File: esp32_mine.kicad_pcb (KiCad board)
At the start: 4 copper layers, 100 x 100 mm, 106 parts, among them J1 USB_C_Receptacle_USB2.0_14P, J3 GPIO, M1 PinHeader_1x02_P2.54mm_Vertic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, M2 PinHeader_1x02_P2.54mm_Vertic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, M3 PinHeader_1x02_P2.54mm_Vertic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, M4 PinHeader_1x02_P2.54mm_Vertic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, Q1 AO3401A, Q2 Q_NMOS_GSD, Q3 Q_NMOS_GSD, Q4 Q_NMOS_GSD, Q5 Q_NMOS_GSD, U1 ESP32-S3, U2 W25Q128JVS, U3 MCP73831-2-OT, U4 BNO055, U5 BMP280, U6 NUP2202, U7 RT9701, Y1 32.768 kHz, Y2 40MHz(10ppm), Y3 32.768 kHz

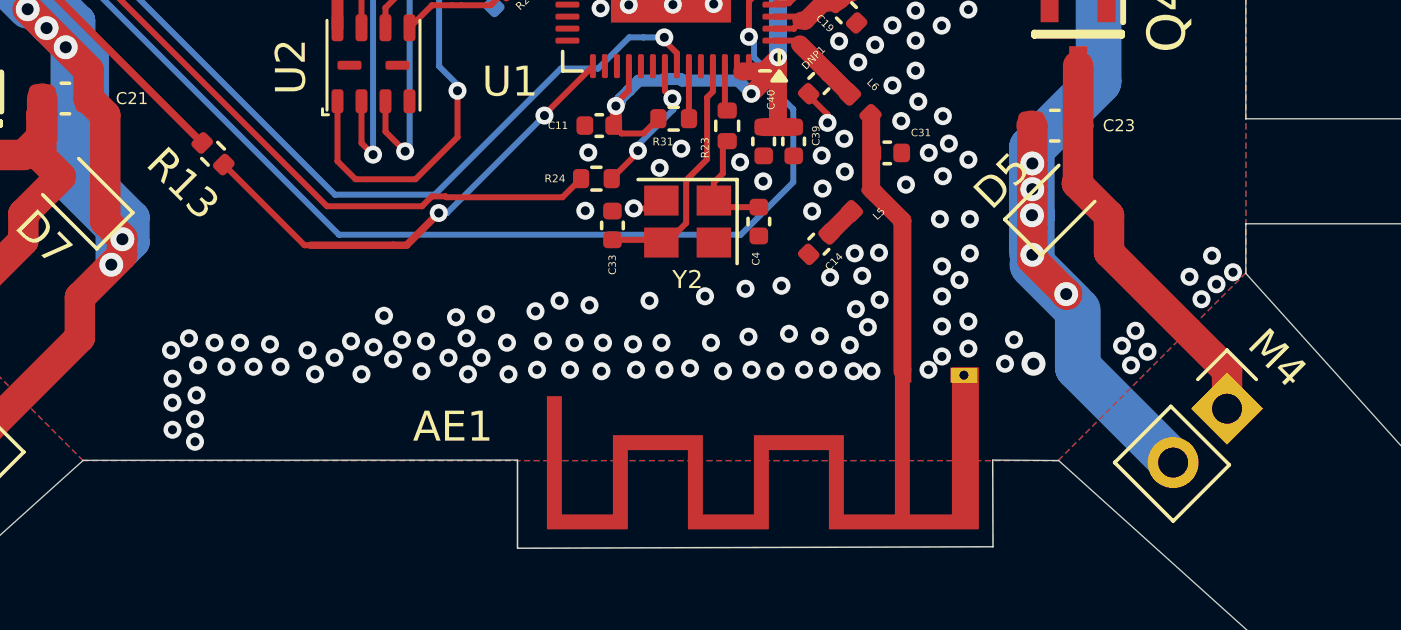
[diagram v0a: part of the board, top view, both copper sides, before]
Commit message: save
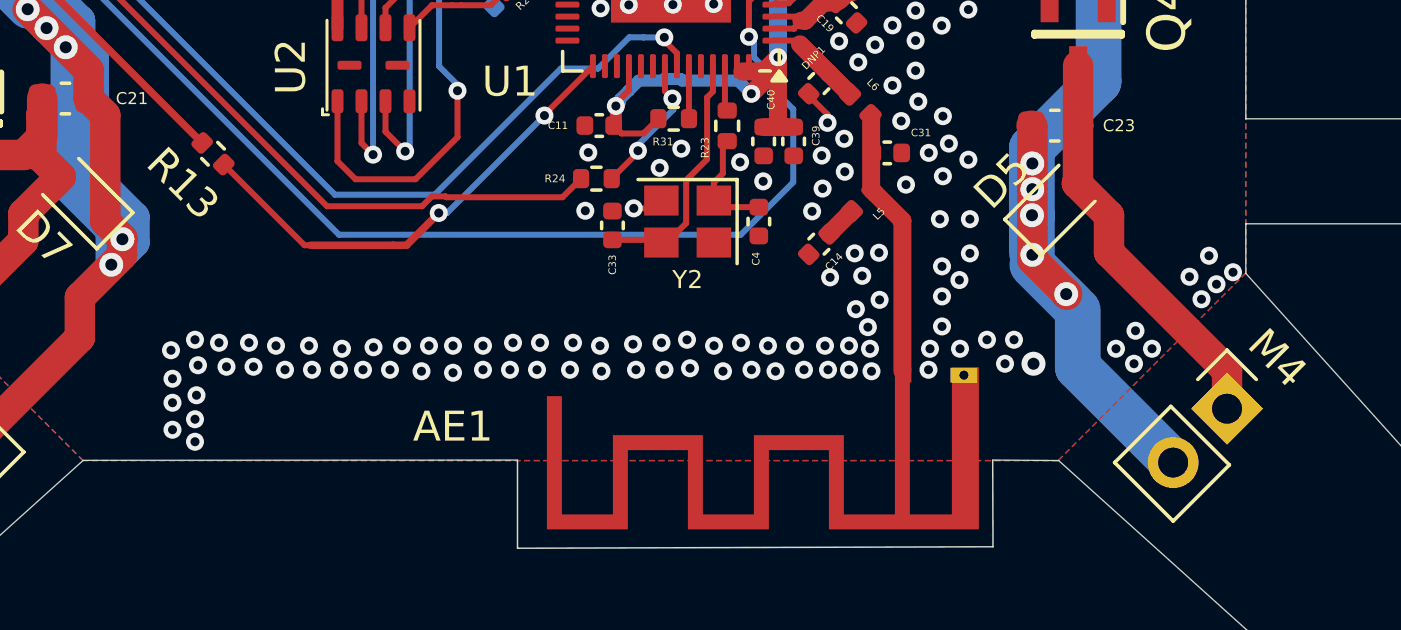
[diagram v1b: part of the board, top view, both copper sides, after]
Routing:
- net GND: vias 208 -> 201
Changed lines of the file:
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@@
 		(filling no)
 		(pcbplotparams
-			(layerselection 0x00000000_00000000_55555555_5755f0af)
+			(layerselection 0x00000000_00000000_55555555_5755f5ff)
 			(plot_on_all_layers_selection 0x00000000_00000000_00000000_00000000)
 			(disableapertmacros no)
-			(usegerberextensions no)
+			(usegerberextensions yes)
 			(usegerberattributes yes)
 			(usegerberadvancedattributes yes)
-			(creategerberjobfile yes)
+			(creategerberjobfile no)
 			(dashed_line_dash_ratio 12)
 			(dashed_line_gap_ratio 3)
@@
 	)
 	(via
-		(at 105.5 115.15)
+		(at 105.4 115.5)
 		(size 0.6)
 		(drill 0.3)
@@
 	)
 	(via
-		(at 124.68 113.89)
+		(at 125.3 114.5)
 		(size 0.6)
 		(drill 0.3)
@@
 	)
 	(via
-		(at 106.6 114.55)
+		(at 106.7 114.7)
 		(size 0.6)
 		(drill 0.3)
@@
 	)
 	(via
-		(at 111.55 114.6)
+		(at 111.5 114.6)
 		(size 0.6)
 		(drill 0.3)
@@
 	)
 	(via
-		(at 102.9 115.65)
+		(at 102.8 115.5)
 		(size 0.6)
 		(drill 0.3)
@@
 	)
 	(via
-		(at 108 115.65)
+		(at 107.5 115.6)
 		(size 0.6)
 		(drill 0.3)
@@
 	)
 	(via
-		(at 117.35 114.4)
+		(at 117.1 114.6)
 		(size 0.6)
 		(drill 0.3)
@@
 	)
 	(via
-		(at 110.25 113.55)
-		(size 0.6)
-		(drill 0.3)
-		(layers "F.Cu" "B.Cu")
-		(free yes)
-		(capping no)
-		(covering
-			(front no)
-			(back no)
-		)
-		(plugging
-			(front no)
-			(back no)
-		)
-		(filling no)
-		(net "GND")
-	)
-	(via
 		(at 106.45 115.55)
 		(size 0.6)
@@
 	)
 	(via
-		(at 112.5 114.6)
+		(at 112.4 114.7)
 		(size 0.6)
 		(drill 0.3)
@@
 	)
 	(via
-		(at 112.05 113.35)
-		(size 0.6)
-		(drill 0.3)
-		(layers "F.Cu" "B.Cu")
-		(free yes)
-		(capping no)
-		(covering
-			(front no)
-			(back no)
-		)
-		(plugging
-			(front no)
-			(back no)
-		)
-		(filling no)
-		(net "GND")
-	)
-	(via
 		(at 124.68 100.489615)
 		(size 0.6)
@@
 	)
 	(via
-		(at 111.05 113.2)
-		(size 0.6)
-		(drill 0.3)
-		(layers "F.Cu" "B.Cu")
-		(free yes)
-		(capping no)
-		(covering
-			(front no)
-			(back no)
-		)
-		(plugging
-			(front no)
-			(back no)
-		)
-		(filling no)
-		(net "GND")
-	)
-	(via
-		(at 101.4 114.65)
+		(at 101.6 114.7)
 		(size 0.6)
 		(drill 0.3)
@@
 	)
 	(via
-		(at 100.4 114.6)
+		(at 100.7 114.6)
 		(size 0.6)
 		(drill 0.3)
@@
 	)
 	(via
-		(at 109.35 115.65)
-		(size 0.6)
-		(drill 0.3)
-		(layers "F.Cu" "B.Cu")
-		(free yes)
-		(capping no)
-		(covering
-			(front no)
-			(back no)
-		)
-		(plugging
-			(front no)
-			(back no)
-		)
-		(filling no)
-		(net "GND")
-	)
-	(via
-		(at 115.9 113.05)
+		(at 109.4 115.5)
 		(size 0.6)
 		(drill 0.3)
@@
 	)
 	(via
-		(at 104.1 114.55)
+		(at 104.5 115.5)
 		(size 0.6)
 		(drill 0.3)
@@
 	)
 	(via
-		(at 107.35 115.1)
+		(at 107.5 114.7)
 		(size 0.6)
 		(drill 0.3)
@@
 	)
 	(via
-		(at 129.8 114.7)
+		(at 129.6 114.8)
 		(size 0.6)
 		(drill 0.3)
@@
 	)
 	(via
-		(at 130.1 115.35)
+		(at 130.2 115.3)
 		(size 0.6)
 		(drill 0.3)
@@
 	)
 	(via
-		(at 110.5 114.55)
+		(at 110.4 114.6)
 		(size 0.6)
 		(drill 0.3)
@@
 	)
 	(via
-		(at 114.05 113.2)
+		(at 115.3 114.5)
 		(size 0.6)
 		(drill 0.3)
@@
 	)
 	(via
-		(at 103.55 115.1)
+		(at 103.8 114.8)
 		(size 0.6)
 		(drill 0.3)
@@
 	)
 	(via
-		(at 123.8 115.057693)
+		(at 123.4 114.8)
 		(size 0.6)
 		(drill 0.3)
@@
 	)
 	(via
-		(at 99.55 114.6)
+		(at 99.7 114.6)
 		(size 0.6)
 		(drill 0.3)
@@
 	)
 	(via
-		(at 105.8 114.5)
+		(at 105.8 114.7)
 		(size 0.6)
 		(drill 0.3)
@@
 	)
 	(via
-		(at 108.6 113.65)
-		(size 0.6)
-		(drill 0.3)
-		(layers "F.Cu" "B.Cu")
-		(free yes)
-		(capping no)
-		(covering
-			(front no)
-			(back no)
-		)
-		(plugging
-			(front no)
-			(back no)
-		)
-		(filling no)
-		(net "GND")
-	)
-	(via
-		(at 120.85 115.55)
+		(at 120.7 115.5)
 		(size 0.6)
 		(drill 0.3)
@@
 	)
 	(via
-		(at 104.45 115.65)
+		(at 103.7 115.5)
 		(size 0.6)
 		(drill 0.3)
@@
 	)
 	(via
-		(at 132.8 111.7)
+		(at 132.7 111.7)
 		(size 0.6)
 		(drill 0.3)
@@
 	)
 	(via
-		(at 117.25 112.8)
+		(at 118 114.7)
 		(size 0.6)
 		(drill 0.3)
@@
 	)
 	(via
-		(at 120.73 114.68)
+		(at 121.4 114.8)
 		(size 0.6)
 		(drill 0.3)
@@
 	)
 	(via
-		(at 105.2 113.7)
-		(size 0.6)
-		(drill 0.3)
-		(layers "F.Cu" "B.Cu")
-		(free yes)
-		(capping no)
-		(covering
-			(front no)
-			(back no)
-		)
-		(plugging
-			(front no)
-			(back no)
-		)
-		(filling no)
-		(net "GND")
-	)
-	(via
 		(at 110.5416 87.2233)
 		(size 0.6)
@@
 	)
 	(via
-		(at 119.73 114.38)
+		(at 119.9 114.7)
 		(size 0.6)
 		(drill 0.3)
@@
 	)
 	(via
-		(at 118.45 112.7)
+		(at 120.7 114.7)
 		(size 0.6)
 		(drill 0.3)
@@
 	)
 	(via
-		(at 118.7 114.3)
+		(at 118.9 114.7)
 		(size 0.6)
 		(drill 0.3)
@@
 	)
 	(via
-		(at 116.1 114.6)
+		(at 116.2 114.7)
 		(size 0.6)
 		(drill 0.3)
@@
 	)
 	(via
-		(at 124.68 114.795)
+		(at 124.4 114.8)
 		(size 0.6)
 		(drill 0.3)
@@
 	)
 	(via
-		(at 98.7 114.45)
+		(at 98.9 114.5)
 		(size 0.6)
 		(drill 0.3)
@@
 	)
 	(via
-		(at 108.45 115.1)
+		(at 108.5 115.5)
 		(size 0.6)
 		(drill 0.3)
@@
 	)
 	(via
-		(at 107.6 113.75)
-		(size 0.6)
-		(drill 0.3)
-		(layers "F.Cu" "B.Cu")
-		(free yes)
-		(capping no)
-		(covering
-			(front no)
-			(back no)
-		)
-		(plugging
-			(front no)
-			(back no)
-		)
-		(filling no)
-		(net "GND")
-	)
-	(via
 		(at 121.33 114.08)
 		(size 0.6)
@@
 	)
 	(via
-		(at 101.75 115.4)
+		(at 101.9 115.5)
 		(size 0.6)
 		(drill 0.3)
@@
 	)
 	(via
-		(at 130.65 114.9)
+		(at 130.8 114.8)
 		(size 0.6)
 		(drill 0.3)
@@
 	)
 	(via
-		(at 107.95 114.45)
+		(at 108.5 114.7)
 		(size 0.6)
 		(drill 0.3)
@@
 	)
 	(via
-		(at 102.65 114.85)
+		(at 102.7 114.7)
 		(size 0.6)
 		(drill 0.3)
@@
 	)
 	(via
-		(at 109.3 114.6)
+		(at 109.5 114.6)
 		(size 0.6)
 		(drill 0.3)
